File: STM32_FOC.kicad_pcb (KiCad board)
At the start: 4 copper layers, 26.5 x 26.5 mm, 47 parts, among them J1 Conn_01x04, J2 Conn_01x02, J3 Conn_01x03, J4 Conn_01x04, J5 Conn_01x06, U1 STM32F103C8T6, U2 MP2359, U3 AS5600, U4 DRV8313, Y1 Crystal_GND3_Small

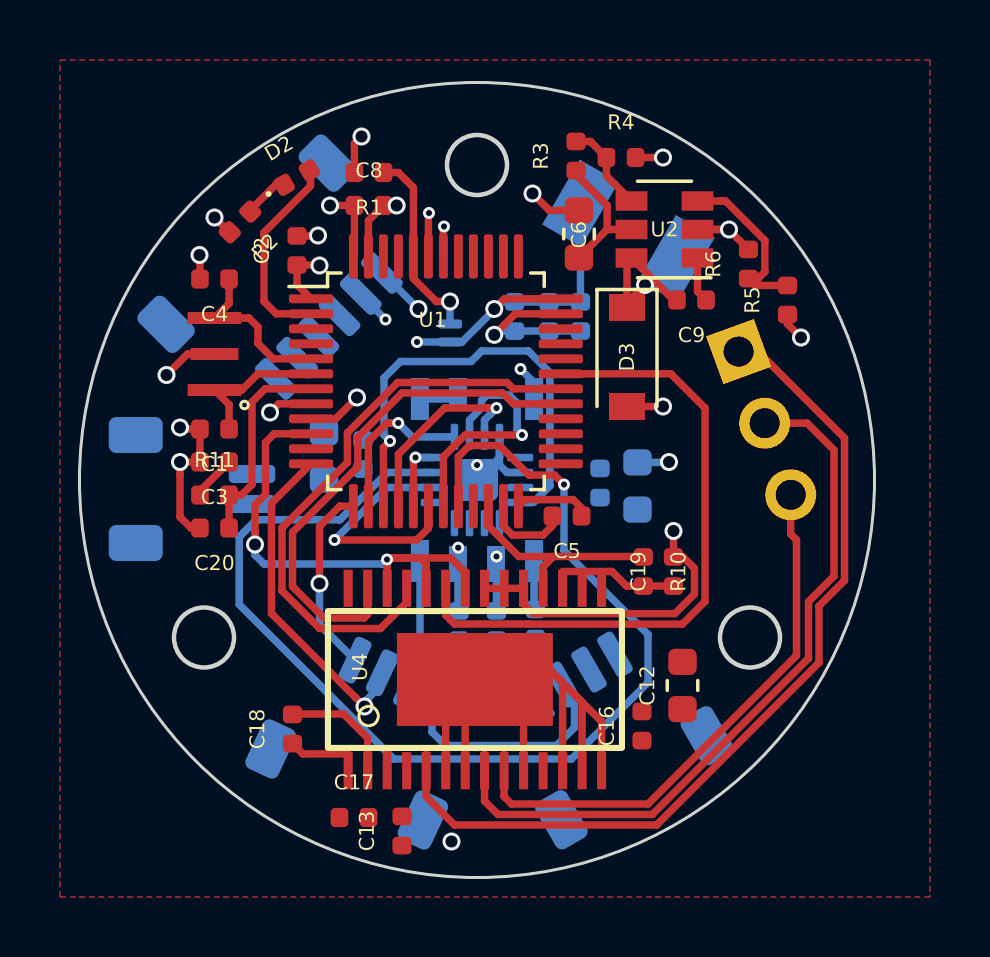
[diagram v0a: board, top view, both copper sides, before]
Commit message: update
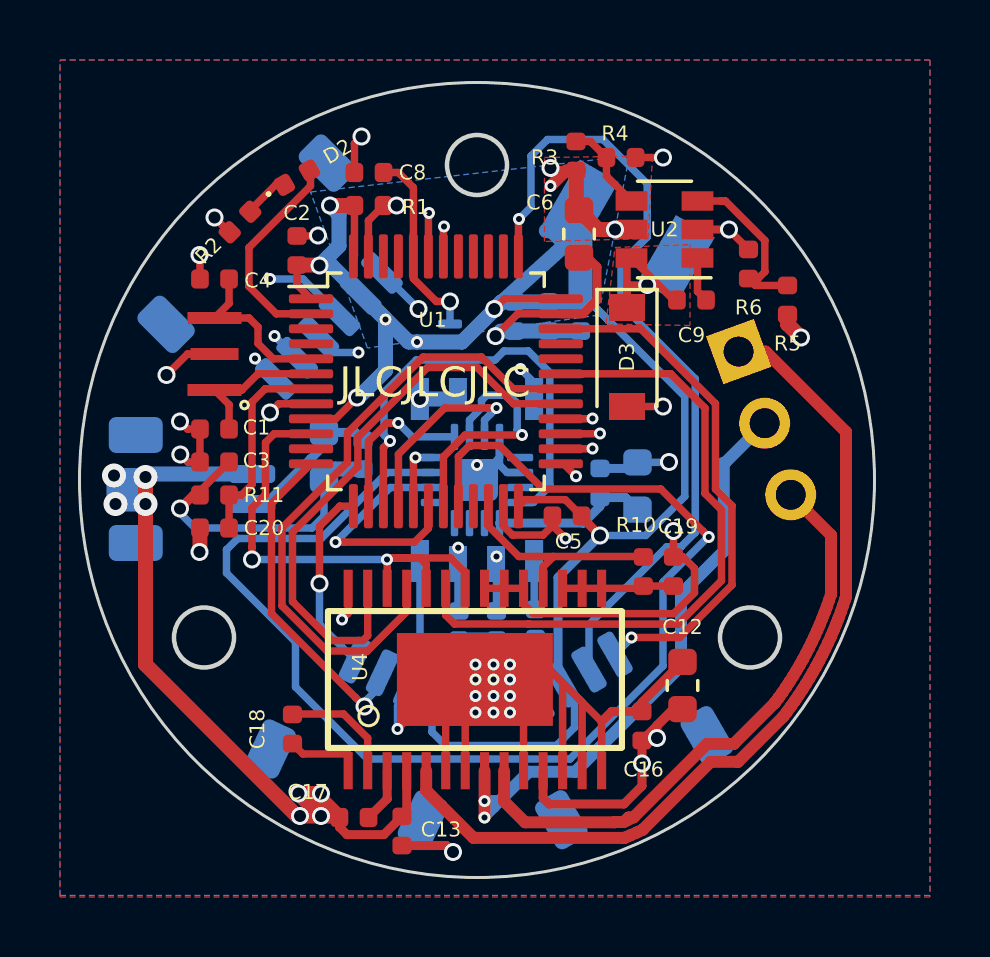
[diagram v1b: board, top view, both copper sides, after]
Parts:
- turned C17 to 180 degrees
- turned C21 to 90 degrees
- turned C6 to 270 degrees
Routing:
- net +12V: track 4.53 -> 84.2 mm, vias 0 -> 13
- net +3V3: track 38.5 -> 108.7 mm, vias 7 -> 10
- net SWCLK: track 0.00 -> 27.6 mm, vias 0 -> 1
- net SPI2_SCK: track 0.00 -> 24.3 mm, vias 0 -> 2
- net SPI2_CS: track 0.00 -> 24.2 mm, vias 0 -> 2
- net SPI2_MISO: track 0.00 -> 23.3 mm, vias 0 -> 2
- net SPI2_MOSI: track 0.00 -> 21.1 mm, vias 0 -> 2
- net SWDIO: track 0.00 -> 17.3 mm, vias 0 -> 1
- net GND: track 85.7 -> 102.3 mm, vias 20 -> 35
- net Net-(C21-Pad1): track 0.00 -> 5.29 mm
- net V: track 24.7 -> 20.0 mm, vias 0 -> 2
- net Z: track 40.1 -> 44.4 mm
- net PWMA: track 17.3 -> 19.3 mm
- net PWMB: track 19.6 -> 21.4 mm
- net W: track 18.8 -> 20.1 mm
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- added copper zone on F.Cu, net +12V
- added copper zone on In2.Cu, net +12V
- added copper zone on B.Cu, net +3V3
- added copper zone on In2.Cu, net +3V3
- added copper zone on B.Cu, net GND
- added copper zone on F.Cu, net Net-(C9-Pad2)
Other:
- board text added: "JLCJLCJLC"

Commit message: update
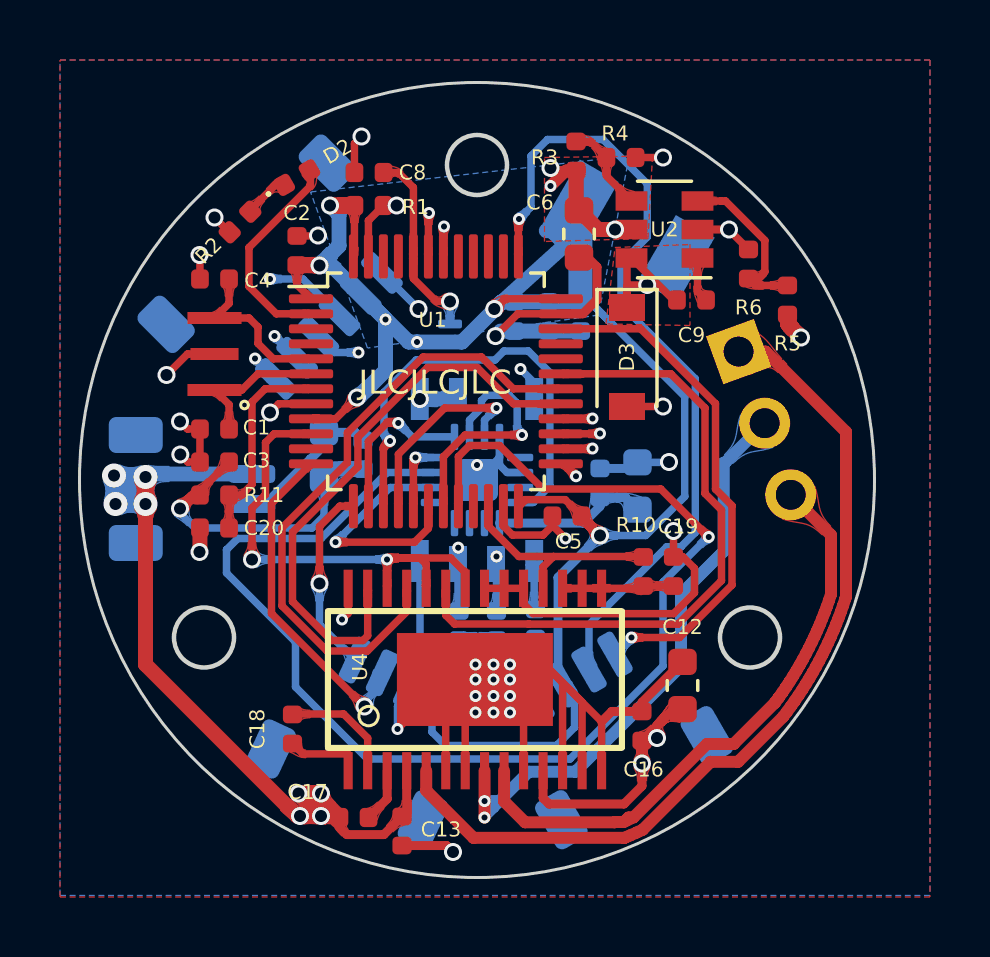
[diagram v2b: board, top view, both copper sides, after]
